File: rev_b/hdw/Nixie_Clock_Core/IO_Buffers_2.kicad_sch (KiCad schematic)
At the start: 14 parts

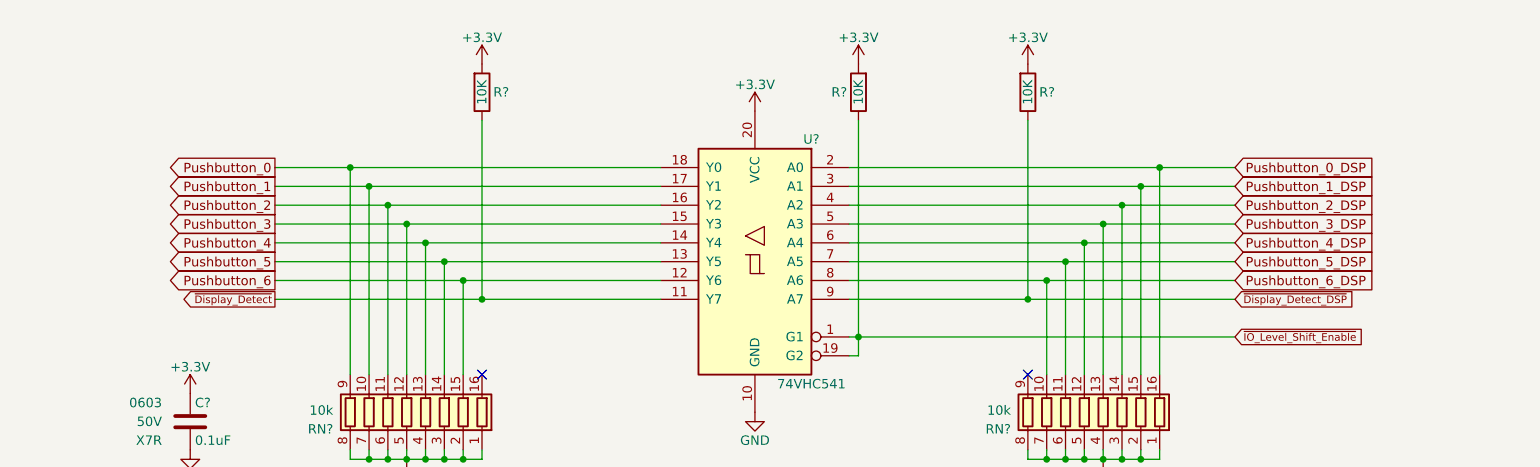
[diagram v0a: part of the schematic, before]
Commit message: lots more PCB placement
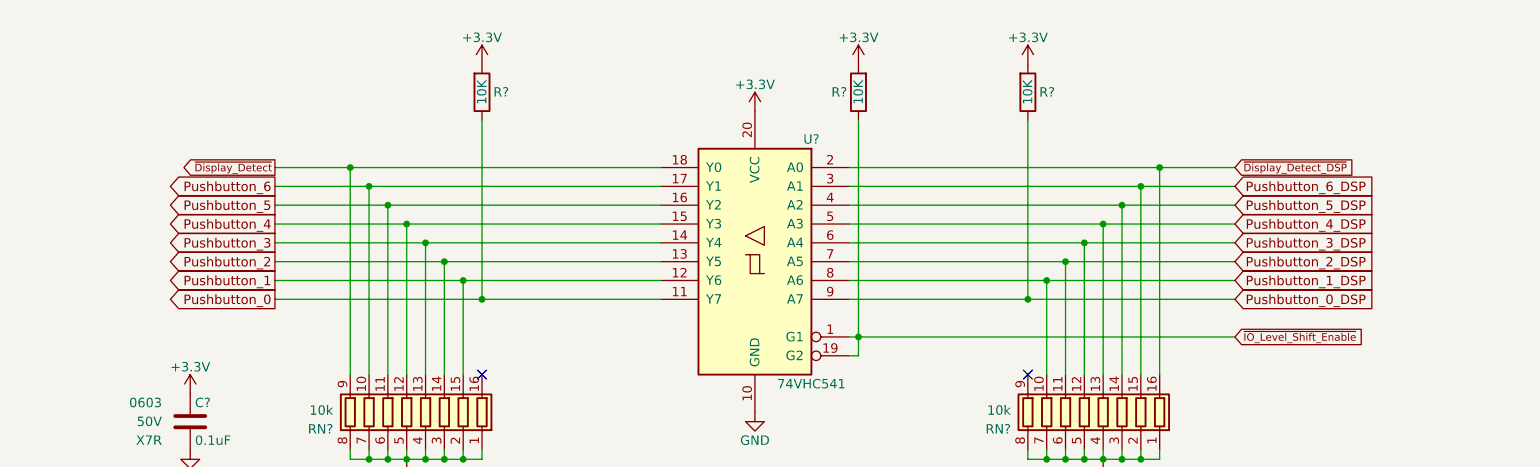
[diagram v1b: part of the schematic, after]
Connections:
- net Pushbutton_0: now also R?.2, U?.11 (Y7); no longer RN?.9 (R8.2), U?.18 (Y0)
- net Pushbutton_0_DSP: now also R?.2, U?.9 (A7); no longer RN?.16 (R1.2), U?.2 (A0)
- net Pushbutton_1: now also RN?.15 (R2.2), U?.12 (Y6); no longer RN?.10 (R7.2), U?.17 (Y1)
- net Pushbutton_1_DSP: now also RN?.10 (R7.2), U?.8 (A6); no longer RN?.15 (R2.2), U?.3 (A1)
- net Pushbutton_2: now also RN?.14 (R3.2), U?.13 (Y5); no longer RN?.11 (R6.2), U?.16 (Y2)
- net Pushbutton_2_DSP: now also RN?.11 (R6.2), U?.7 (A5); no longer RN?.14 (R3.2), U?.4 (A2)
- net Pushbutton_3: now also RN?.13 (R4.2), U?.14 (Y4); no longer RN?.12 (R5.2), U?.15 (Y3)
- net Pushbutton_3_DSP: now also RN?.12 (R5.2), U?.6 (A4); no longer RN?.13 (R4.2), U?.5 (A3)
- net Pushbutton_4: now also RN?.12 (R5.2), U?.15 (Y3); no longer RN?.13 (R4.2), U?.14 (Y4)
- net Pushbutton_4_DSP: now also RN?.13 (R4.2), U?.5 (A3); no longer RN?.12 (R5.2), U?.6 (A4)
- net Pushbutton_5: now also RN?.11 (R6.2), U?.16 (Y2); no longer RN?.14 (R3.2), U?.13 (Y5)
- net Pushbutton_5_DSP: now also RN?.14 (R3.2), U?.4 (A2); no longer RN?.11 (R6.2), U?.7 (A5)
- net Pushbutton_6: now also RN?.10 (R7.2), U?.17 (Y1); no longer RN?.15 (R2.2), U?.12 (Y6)
- net Pushbutton_6_DSP: now also RN?.15 (R2.2), U?.3 (A1); no longer RN?.10 (R7.2), U?.8 (A6)
- net ~{Display_Detect_DSP}: now also RN?.16 (R1.2), U?.2 (A0); no longer R?.2, U?.9 (A7)
- net ~{Display_Detect}: now also RN?.9 (R8.2), U?.18 (Y0); no longer R?.2, U?.11 (Y7)
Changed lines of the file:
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@@
     (effects (font (face "Courier New") (size 5.08 5.08) (thickness 0.254) bold (color 255 37 56 1)) (justify left bottom))
   )
-  (global_label "Pushbutton_2" (shape output) (at 64.77 111.76 180) (fields_autoplaced)
+  (global_label "Pushbutton_2" (shape output) (at 64.77 119.38 180) (fields_autoplaced)
+    (effects (font (size 1.27 1.27)) (justify right))
+    (property "Intersheetrefs" "${INTERSHEET_REFS}" (at 49.0436 119.38 0)
+      (effects (font (size 1.27 1.27)) (justify right) hide)
+    )
+  )
+  (global_label "Pushbutton_5" (shape output) (at 64.77 111.76 180) (fields_autoplaced)
     (effects (font (size 1.27 1.27)) (justify right))
     (property "Intersheetrefs" "${INTERSHEET_REFS}" (at 49.0436 111.76 0)
@@
     )
   )
-  (global_label "Pushbutton_5" (shape output) (at 64.77 119.38 180) (fields_autoplaced)
-    (effects (font (size 1.27 1.27)) (justify right))
-    (property "Intersheetrefs" "${INTERSHEET_REFS}" (at 49.0436 119.38 0)
-      (effects (font (size 1.27 1.27)) (justify right) hide)
-    )
-  )
-  (global_label "~{Display_Detect_DSP}" (shape input) (at 194.31 124.46 0)
+  (global_label "~{Display_Detect_DSP}" (shape input) (at 194.31 106.68 0)
     (effects (font (size 1.016 1.016)) (justify left))
-    (property "Intersheetrefs" "${INTERSHEET_REFS}" (at 194.31 124.46 0)
+    (property "Intersheetrefs" "${INTERSHEET_REFS}" (at 194.31 106.68 0)
       (effects (font (size 1.27 1.27)) hide)
     )
   )
-  (global_label "Pushbutton_6_DSP" (shape input) (at 194.31 121.92 0) (fields_autoplaced)
+  (global_label "Pushbutton_6_DSP" (shape input) (at 194.31 109.22 0) (fields_autoplaced)
     (effects (font (size 1.27 1.27)) (justify left))
-    (property "Intersheetrefs" "${INTERSHEET_REFS}" (at 214.7535 121.92 0)
+    (property "Intersheetrefs" "${INTERSHEET_REFS}" (at 214.7535 109.22 0)
       (effects (font (size 1.27 1.27)) (justify left) hide)
     )
@@
     )
   )
-  (global_label "Pushbutton_6" (shape output) (at 64.77 121.92 180) (fields_autoplaced)
+  (global_label "Pushbutton_6" (shape output) (at 64.77 109.22 180) (fields_autoplaced)
     (effects (font (size 1.27 1.27)) (justify right))
-    (property "Intersheetrefs" "${INTERSHEET_REFS}" (at 49.0436 121.92 0)
+    (property "Intersheetrefs" "${INTERSHEET_REFS}" (at 49.0436 109.22 0)
       (effects (font (size 1.27 1.27)) (justify right) hide)
     )
   )
-  (global_label "Pushbutton_2_DSP" (shape input) (at 194.31 111.76 0) (fields_autoplaced)
+  (global_label "Pushbutton_2_DSP" (shape input) (at 194.31 119.38 0) (fields_autoplaced)
     (effects (font (size 1.27 1.27)) (justify left))
-    (property "Intersheetrefs" "${INTERSHEET_REFS}" (at 214.7535 111.76 0)
+    (property "Intersheetrefs" "${INTERSHEET_REFS}" (at 214.7535 119.38 0)
       (effects (font (size 1.27 1.27)) (justify left) hide)
     )
   )
-  (global_label "~{Display_Detect}" (shape output) (at 64.77 124.46 180)
+  (global_label "~{Display_Detect}" (shape output) (at 64.77 106.68 180)
     (effects (font (size 1.016 1.016)) (justify right))
-    (property "Intersheetrefs" "${INTERSHEET_REFS}" (at 64.77 124.46 0)
+    (property "Intersheetrefs" "${INTERSHEET_REFS}" (at 64.77 106.68 0)
       (effects (font (size 1.27 1.27)) hide)
     )
@@
     )
   )
-  (global_label "Pushbutton_4" (shape output) (at 64.77 116.84 180) (fields_autoplaced)
+  (global_label "Pushbutton_4" (shape output) (at 64.77 114.3 180) (fields_autoplaced)
     (effects (font (size 1.27 1.27)) (justify right))
-    (property "Intersheetrefs" "${INTERSHEET_REFS}" (at 49.0436 116.84 0)
+    (property "Intersheetrefs" "${INTERSHEET_REFS}" (at 49.0436 114.3 0)
       (effects (font (size 1.27 1.27)) (justify right) hide)
     )
   )
-  (global_label "Pushbutton_0" (shape output) (at 64.77 106.68 180) (fields_autoplaced)
+  (global_label "Pushbutton_0" (shape output) (at 64.77 124.46 180) (fields_autoplaced)
     (effects (font (size 1.27 1.27)) (justify right))
-    (property "Intersheetrefs" "${INTERSHEET_REFS}" (at 49.0436 106.68 0)
+    (property "Intersheetrefs" "${INTERSHEET_REFS}" (at 49.0436 124.46 0)
       (effects (font (size 1.27 1.27)) (justify right) hide)
     )
   )
-  (global_label "Pushbutton_1" (shape output) (at 64.77 109.22 180) (fields_autoplaced)
+  (global_label "Pushbutton_1" (shape output) (at 64.77 121.92 180) (fields_autoplaced)
     (effects (font (size 1.27 1.27)) (justify right))
-    (property "Intersheetrefs" "${INTERSHEET_REFS}" (at 49.0436 109.22 0)
+    (property "Intersheetrefs" "${INTERSHEET_REFS}" (at 49.0436 121.92 0)
       (effects (font (size 1.27 1.27)) (justify right) hide)
     )
   )
-  (global_label "Pushbutton_3_DSP" (shape input) (at 194.31 114.3 0) (fields_autoplaced)
+  (global_label "Pushbutton_3_DSP" (shape input) (at 194.31 116.84 0) (fields_autoplaced)
     (effects (font (size 1.27 1.27)) (justify left))
-    (property "Intersheetrefs" "${INTERSHEET_REFS}" (at 214.7535 114.3 0)
+    (property "Intersheetrefs" "${INTERSHEET_REFS}" (at 214.7535 116.84 0)
       (effects (font (size 1.27 1.27)) (justify left) hide)
     )
@@
     )
   )
-  (global_label "Pushbutton_5_DSP" (shape input) (at 194.31 119.38 0) (fields_autoplaced)
+  (global_label "Pushbutton_5_DSP" (shape input) (at 194.31 111.76 0) (fields_autoplaced)
     (effects (font (size 1.27 1.27)) (justify left))
-    (property "Intersheetrefs" "${INTERSHEET_REFS}" (at 214.7535 119.38 0)
+    (property "Intersheetrefs" "${INTERSHEET_REFS}" (at 214.7535 111.76 0)
       (effects (font (size 1.27 1.27)) (justify left) hide)
     )
@@
     )
   )
-  (global_label "Pushbutton_4_DSP" (shape input) (at 194.31 116.84 0) (fields_autoplaced)
+  (global_label "Pushbutton_4_DSP" (shape input) (at 194.31 114.3 0) (fields_autoplaced)
     (effects (font (size 1.27 1.27)) (justify left))
-    (property "Intersheetrefs" "${INTERSHEET_REFS}" (at 214.7535 116.84 0)
+    (property "Intersheetrefs" "${INTERSHEET_REFS}" (at 214.7535 114.3 0)
       (effects (font (size 1.27 1.27)) (justify left) hide)
     )
   )
-  (global_label "Pushbutton_1_DSP" (shape input) (at 194.31 109.22 0) (fields_autoplaced)
+  (global_label "Pushbutton_1_DSP" (shape input) (at 194.31 121.92 0) (fields_autoplaced)
     (effects (font (size 1.27 1.27)) (justify left))
-    (property "Intersheetrefs" "${INTERSHEET_REFS}" (at 214.7535 109.22 0)
+    (property "Intersheetrefs" "${INTERSHEET_REFS}" (at 214.7535 121.92 0)
       (effects (font (size 1.27 1.27)) (justify left) hide)
     )
   )
-  (global_label "Pushbutton_0_DSP" (shape input) (at 194.31 106.68 0) (fields_autoplaced)
+  (global_label "Pushbutton_0_DSP" (shape input) (at 194.31 124.46 0) (fields_autoplaced)
     (effects (font (size 1.27 1.27)) (justify left))
-    (property "Intersheetrefs" "${INTERSHEET_REFS}" (at 214.7535 106.68 0)
+    (property "Intersheetrefs" "${INTERSHEET_REFS}" (at 214.7535 124.46 0)
       (effects (font (size 1.27 1.27)) (justify left) hide)
     )
   )
-  (global_label "Pushbutton_3" (shape output) (at 64.77 114.3 180) (fields_autoplaced)
+  (global_label "Pushbutton_3" (shape output) (at 64.77 116.84 180) (fields_autoplaced)
     (effects (font (size 1.27 1.27)) (justify right))
-    (property "Intersheetrefs" "${INTERSHEET_REFS}" (at 49.0436 114.3 0)
+    (property "Intersheetrefs" "${INTERSHEET_REFS}" (at 49.0436 116.84 0)
       (effects (font (size 1.27 1.27)) (justify right) hide)
     )
